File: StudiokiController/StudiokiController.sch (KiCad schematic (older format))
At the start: 18 parts, among them J1 USB_B_Mini, Q1 Q_DUAL_NPN_NPN_E1B1C2E2B2C1, SW1 SW_Push, SW2 SW_Push, SW3 SW_Push, U1 CH340C, U2 ESP32-WROOM-32D

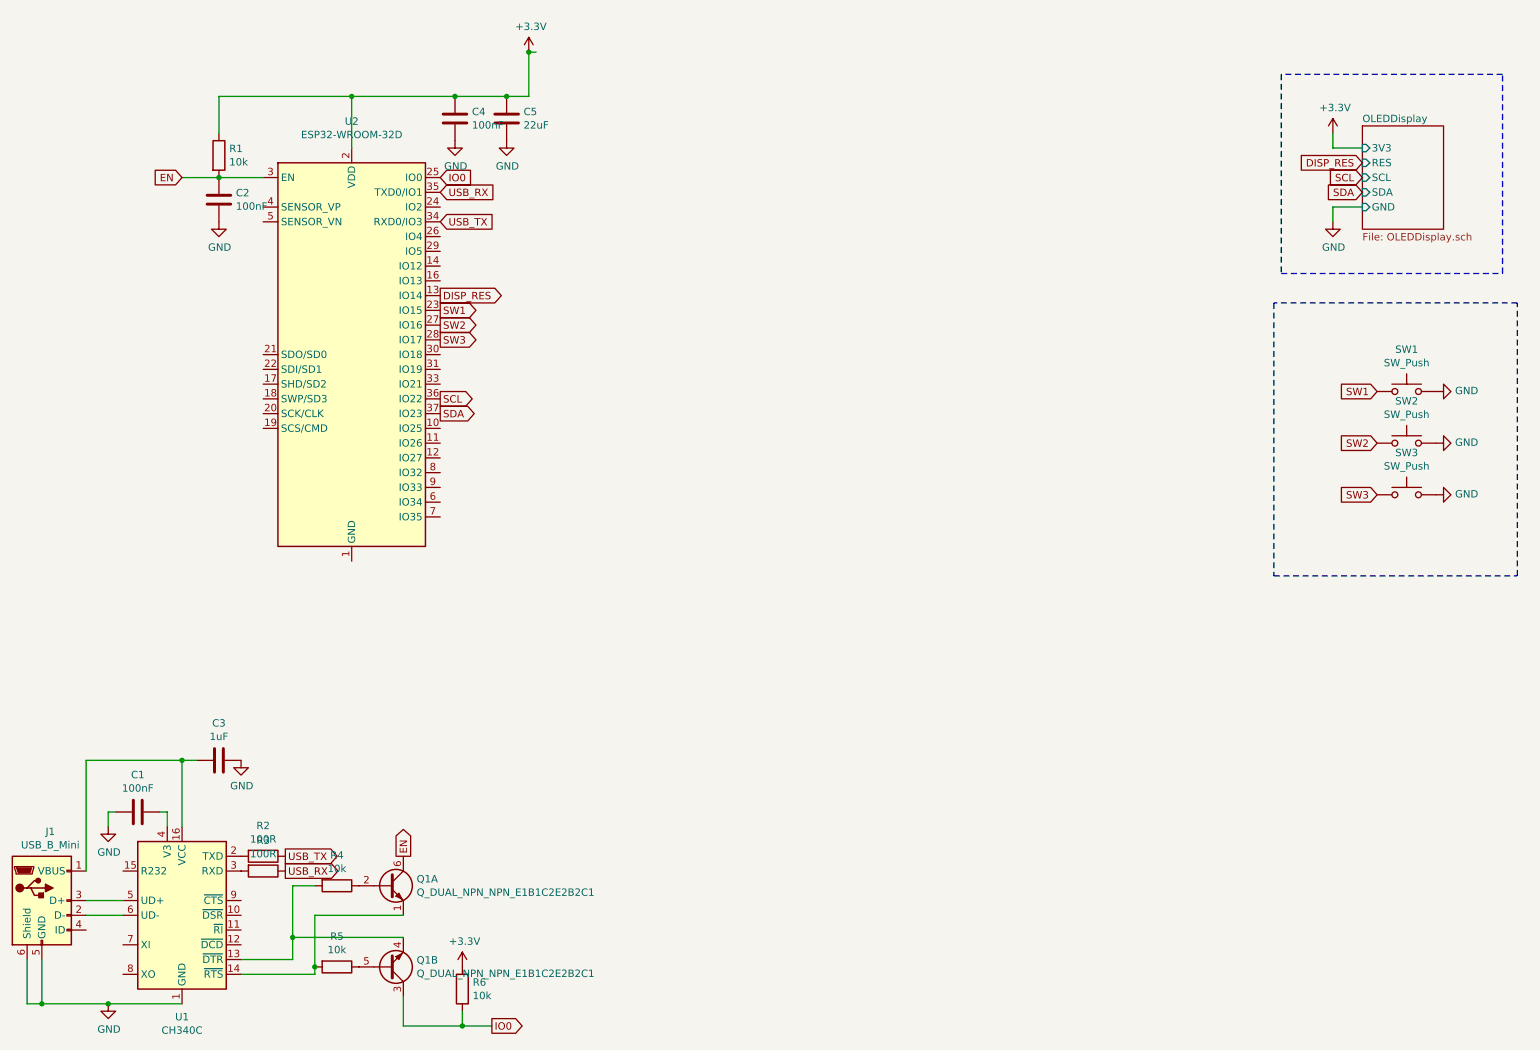
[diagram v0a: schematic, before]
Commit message: Added MAX31855
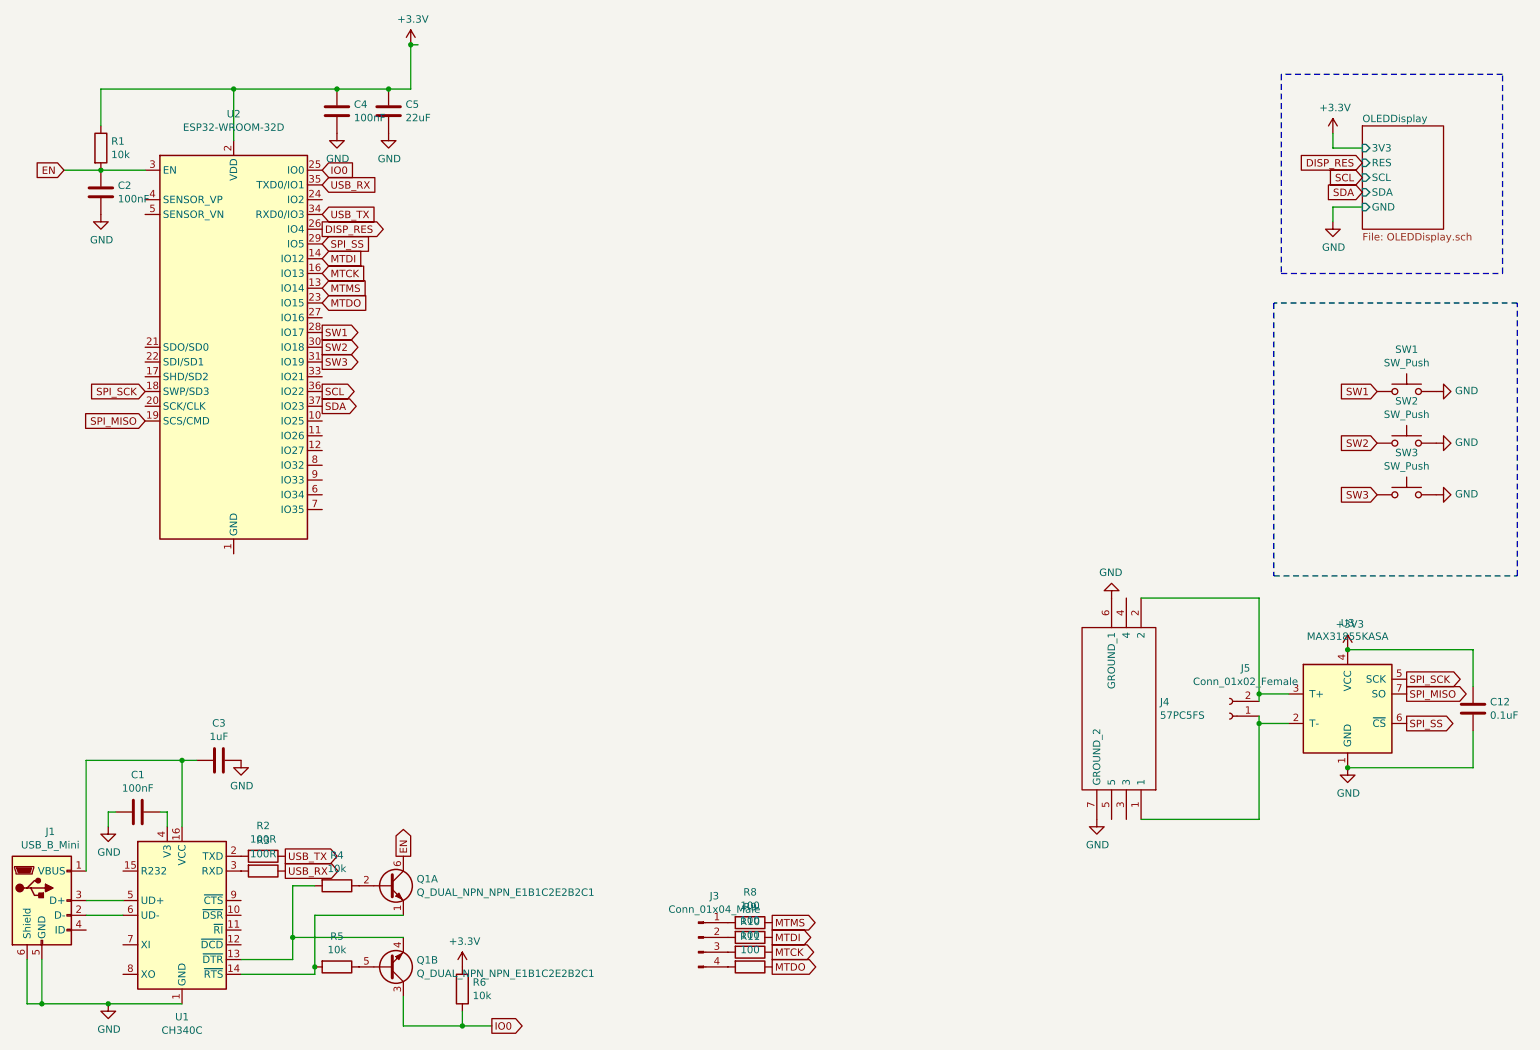
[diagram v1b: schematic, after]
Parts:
- added C12: 0.1uF, Capacitor_SMD:C_0603_1608Metric, symbol Device:C
- added J3: Conn_01x04_Male, Connector_PinHeader_2.54mm:PinHeader_1x04_P2.54mm_Vertical, symbol Connector:Conn_01x04_Male
- added J4: 57PC5FS, 57PC5FS, symbol SamacSys_Parts:57PC5FS
- added J5: Conn_01x02_Female, TerminalBlock:TerminalBlock_bornier-2_P5.08mm, symbol Connector:Conn_01x02_Female
- added R10, R11, R8, R9: 100, Resistor_SMD:R_0603_1608Metric, symbol Device:R
- added U3: MAX31855KASA, Package_SO:SOIC-8_3.9x4.9mm_P1.27mm, symbol Sensor_Temperature:MAX31855KASA
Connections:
- net +3V3: now also C12.1, U3.4 (VCC)
- net DISP_RES: now also U2.26 (IO4); no longer U2.13 (IO14)
- net GND: now also C12.2, J4.6 (GROUND_1), J4.7 (GROUND_2), U3.1 (GND)
- net SW1: now also U2.28 (IO17); no longer U2.23 (IO15)
- net SW2: now also U2.30 (IO18); no longer U2.27 (IO16)
- net SW3: now also U2.31 (IO19); no longer U2.28 (IO17)
- net MTDI: now reaches U2.14 (IO12)
- net MTDI: now also R9.1
- net MTCK: now reaches U2.16 (IO13)
- net MTCK: now also R10.1
- net SPI_SCK: now reaches U2.18 (SWP/SD3)
- net SPI_SCK: now also U3.5 (SCK)
- net SPI_MISO: now reaches U2.19 (SCS/CMD)
- net SPI_MISO: now also U3.7 (SO)
- net SPI_SS: now reaches U2.29 (IO5)
- net SPI_SS: now also U3.6 (~CS~)
- new net: J4.1, J5.1 (Pin_1), U3.2 (T-)
- new net: J4.2, J5.2 (Pin_2), U3.3 (T+)
- new net: J3.1 (Pin_1), R8.2
- new net: J3.2 (Pin_2), R9.2
- new net: J3.3 (Pin_3), R10.2
- new net: J3.4 (Pin_4), R11.2
- new net MTDO: R11.1, U2.23 (IO15)
- new net MTMS: R8.1, U2.13 (IO14)
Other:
- moved on the sheet: C2, C4, C5, R1, U2
